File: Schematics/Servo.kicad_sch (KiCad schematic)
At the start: 8 parts, among them CN1 Limit Switch Connector 1, CN2 Limit Switch Connector 2, J4 Screw_Terminal_01x02, J5 Screw_Terminal_01x02

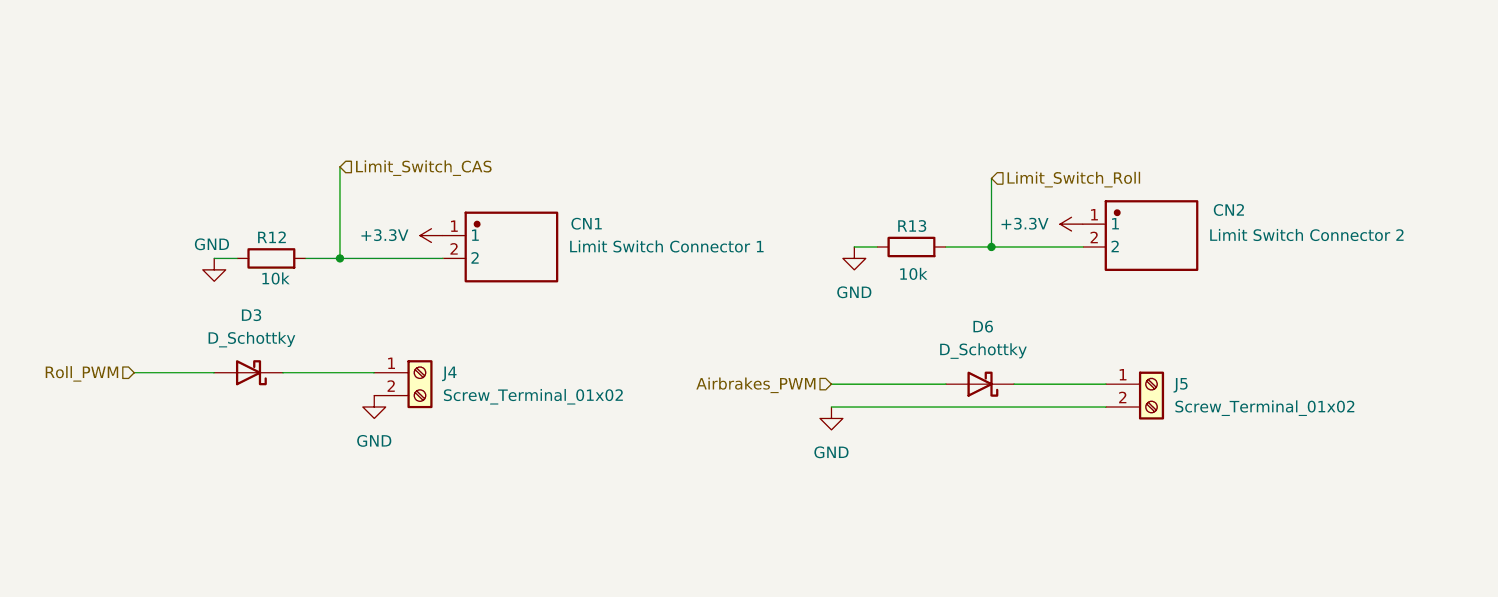
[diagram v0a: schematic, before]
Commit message: final draft, in JLPCB cart
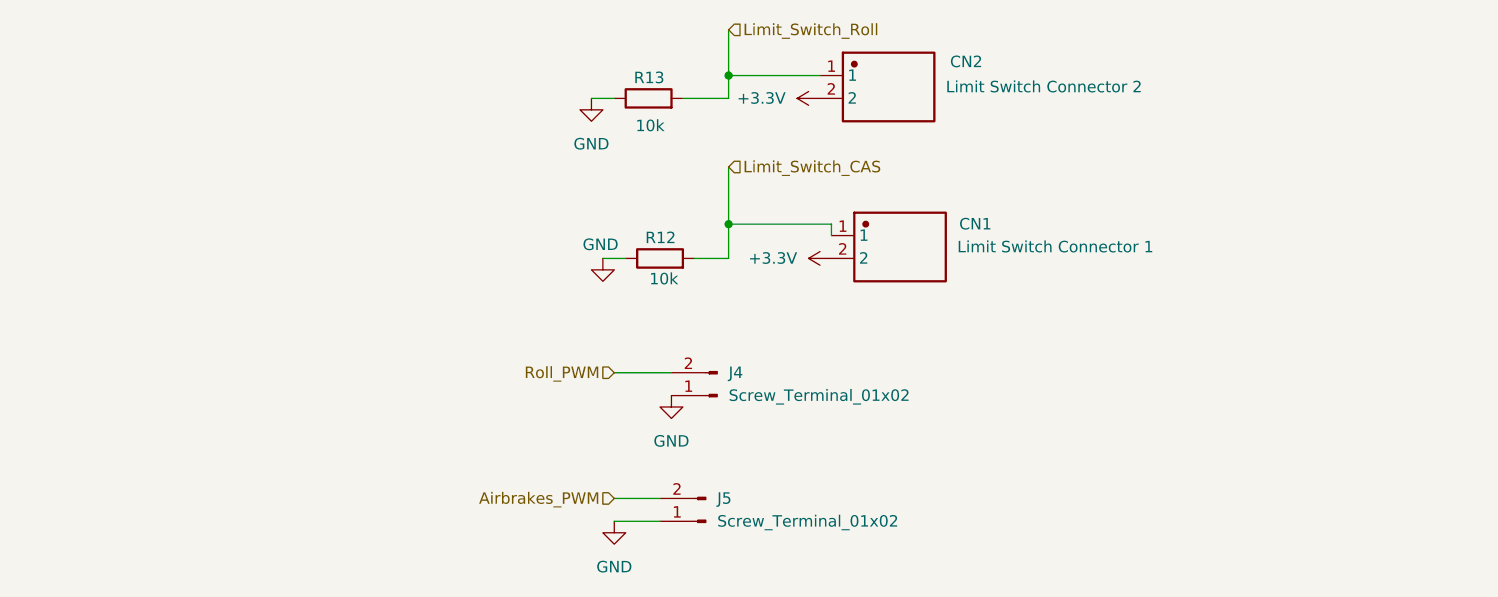
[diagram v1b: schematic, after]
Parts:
- removed D3, D6: D_Schottky, Diode_SMD:D_SOD-123, symbol Device:D_Schottky
- CN1, CN2: footprint myFootprints:JST_B2B-XH-A_LF__SN_ -> Connector_JST:JST_EH_B2B-EH-A_1x02_P2.50mm_Vertical
- J4, J5: footprint Connector_JST:JST_XH_B2B-XH-AM_1x02_P2.50mm_Vertical -> Connector_JST:JST_EH_B2B-EH-A_1x02_P2.50mm_Vertical; symbol Connector:Screw_Terminal_01x02 -> Connector:Conn_01x02_Pin; LCSC C474892 -> C158012
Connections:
- net +3.3V: now also CN1.2, CN2.2; no longer CN1.1, CN2.1
- net Airbrakes_PWM: now also J5.2 (Pin_2)
- net GND: now also J4.1 (Pin_1), J5.1 (Pin_1); no longer J4.2 (Pin_2), J5.2 (Pin_2)
- net Limit_Switch_CAS: now also CN1.1; no longer CN1.2
- net Limit_Switch_Roll: now also CN2.1; no longer CN2.2
- net Roll_PWM: now also J4.2 (Pin_2)
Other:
- moved on the sheet: CN1, CN2, R12, R13
